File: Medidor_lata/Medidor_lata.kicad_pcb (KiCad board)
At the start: 2 copper layers, 7 parts, among them J1 Conn_01x02_Female, SW1 SW_Push, U1 ATmega328P-AU, Y1 Crystal

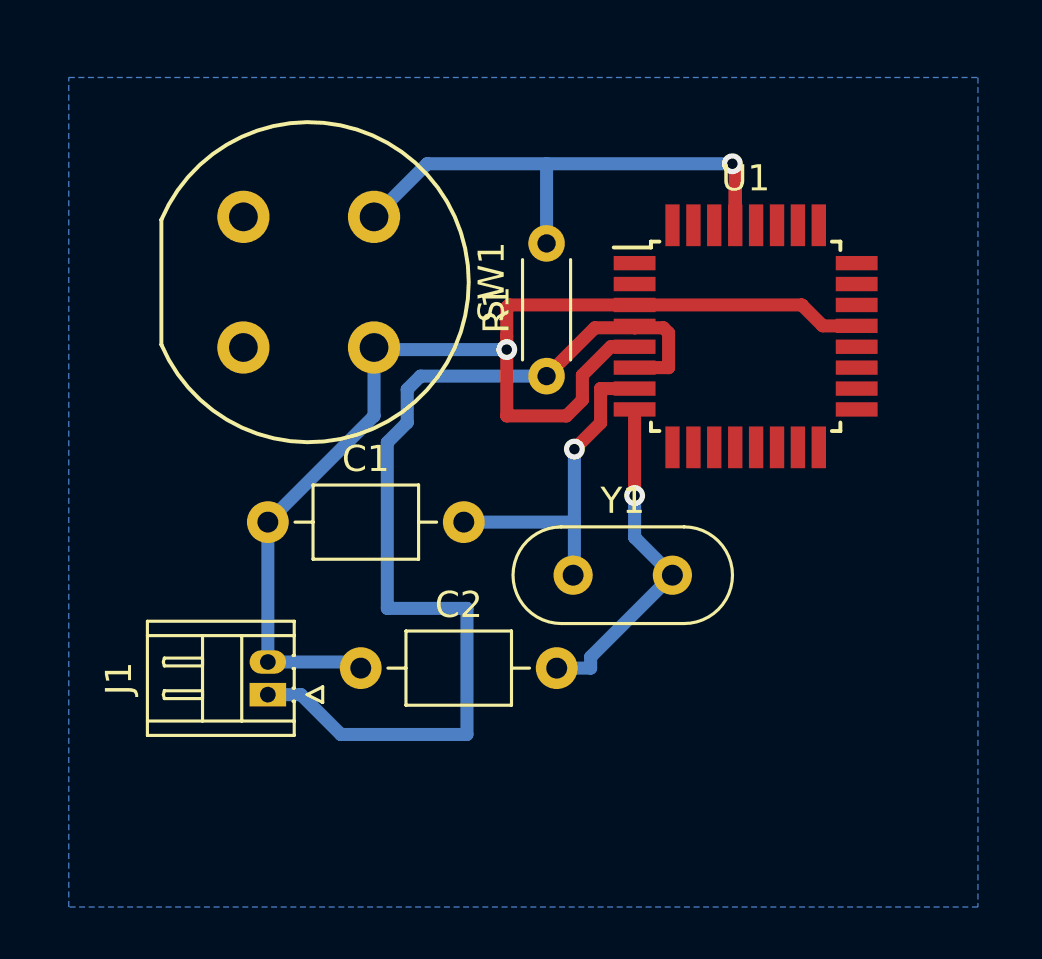
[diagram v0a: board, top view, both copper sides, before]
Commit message: Hemos trabajado en nueva version de sistema de medicio
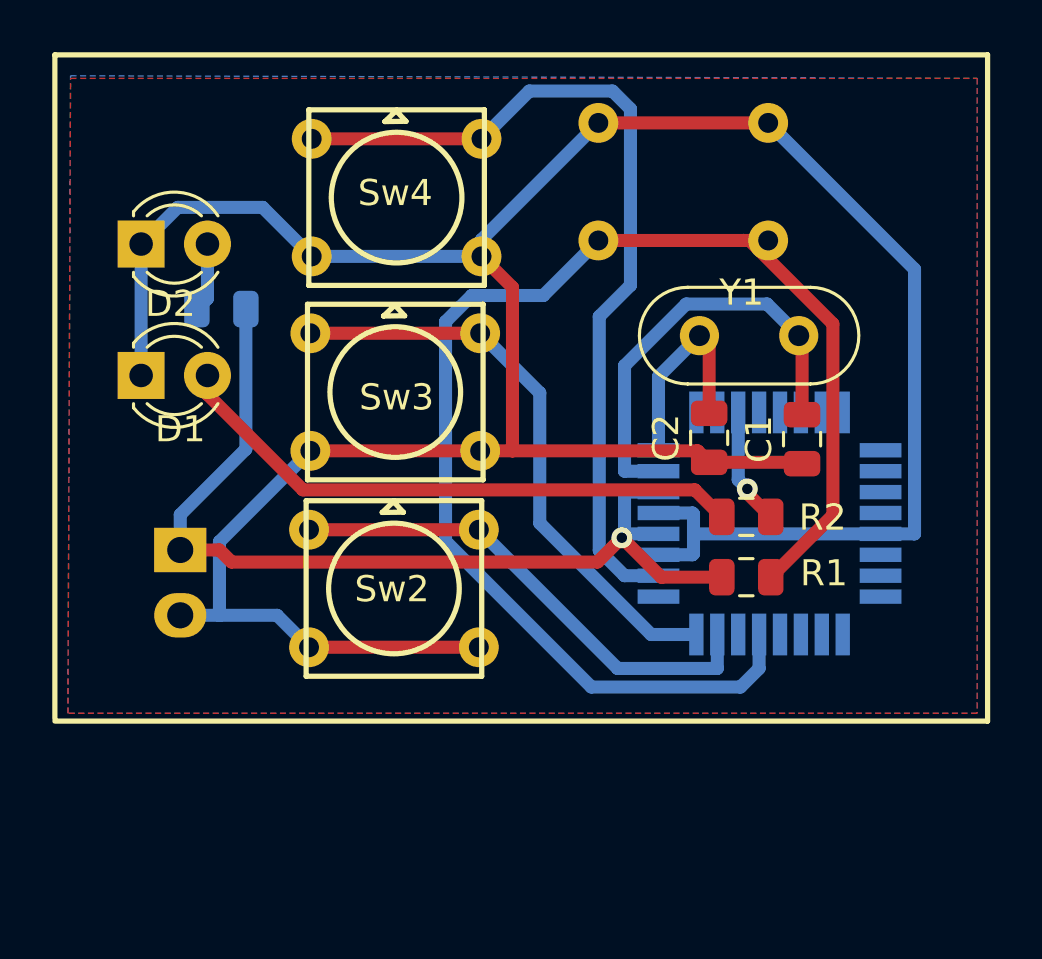
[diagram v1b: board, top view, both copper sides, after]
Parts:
- removed SW1: SW_Push, Button_Switch_THT:Push_E-Switch_KS01Q01
- added D1: LED, LED_THT:LED_D3.0mm, F.Cu at (131.8, 95.0)
- added D2: LED, LED_THT:LED_D3.0mm, F.Cu at (131.8, 89.9)
- added R2: R, Resistor_SMD:R_0805_2012Metric, F.Cu at (155.0, 100.4)
- added R3: R, Resistor_SMD:R_0805_2012Metric, B.Cu at (134.9, 92.4)
- added Sw1: Pulsador, Button_Switch_Keyboard:Pulsador, B.Cu at (152.6, 87.6)
- added Sw2: Pulsador, Button_Switch_Keyboard:Pulsador, F.Cu at (141.5, 103.1)
- added Sw3: Pulsador, Button_Switch_Keyboard:Pulsador, F.Cu at (141.5, 95.6)
- added Sw4: Pulsador, Button_Switch_Keyboard:Pulsador, F.Cu at (141.6, 88.2)
- C1, C2: footprint Capacitor_THT:C_Axial_L3.8mm_D2.6mm_P7.50mm_Horizontal -> Capacitor_SMD:C_0805_2012Metric
- J1: footprint Connector_Hirose:Hirose_DF13-02P-1.25DS_1x02_P1.25mm_Horizontal -> Connector_JST:JST_EH_B02B-EH-A_1x02_P2.50mm_Vertical; moved to B.Cu
- R1: footprint Resistor_THT:R_Axial_DIN0204_L3.6mm_D1.6mm_P5.08mm_Horizontal -> Resistor_SMD:R_0805_2012Metric
- U1: moved to B.Cu
- moved C1 20.7 mm to (157.1, 97.4), turned to 90 degrees
- moved C2 16.0 mm to (153.5, 97.4), turned to 90 degrees
- moved Y1 12.6 mm to (157.0, 93.4), turned to 180 degrees
- moved R1 10.8 mm to (155.0, 102.7), turned to 0 degrees
- moved U1 7.22 mm to (155.9, 100.6)
- moved J1 6.47 mm to (133.3, 101.7), turned to 270 degrees
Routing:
- net GND: track 47.3 -> 110.3 mm, vias 1 -> 0
- net Net-(Sw4-Pad1): track 0.00 -> 33.3 mm
- net Net-(R1-Pad2): track 21.3 -> 53.4 mm, vias 1 -> 0
- net Net-(Sw3-Pad1): track 0.00 -> 22.5 mm
- net Net-(D1-Pad2): track 0.00 -> 22.4 mm
- net Net-(Sw2-Pad1): track 0.00 -> 19.1 mm
- net Net-(C2-Pad2): track 13.1 -> 8.17 mm, vias 1 -> 0
- net Net-(R2-Pad2): track 0.00 -> 4.51 mm, vias 0 -> 1
- net Net-(C1-Pad2): track 13.1 -> 16.6 mm, vias 1 -> 0
- net Net-(D2-Pad2): track 0.00 -> 2.66 mm
- net +5V: track 38.6 -> 36.6 mm, vias 0 -> 1
- added copper zone on F.Cu, net GND
